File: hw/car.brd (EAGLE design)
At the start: 100 x 80 mm, 27 parts, among them Q1 BS170, Q2 BS170, Q3 BS170, Q4 BS170, Q5 BS170, Q6 BS170, Q7 BS170, Q8 BS170, X0 pwm_board, X1 22-23-2041, X3 22-23-2041

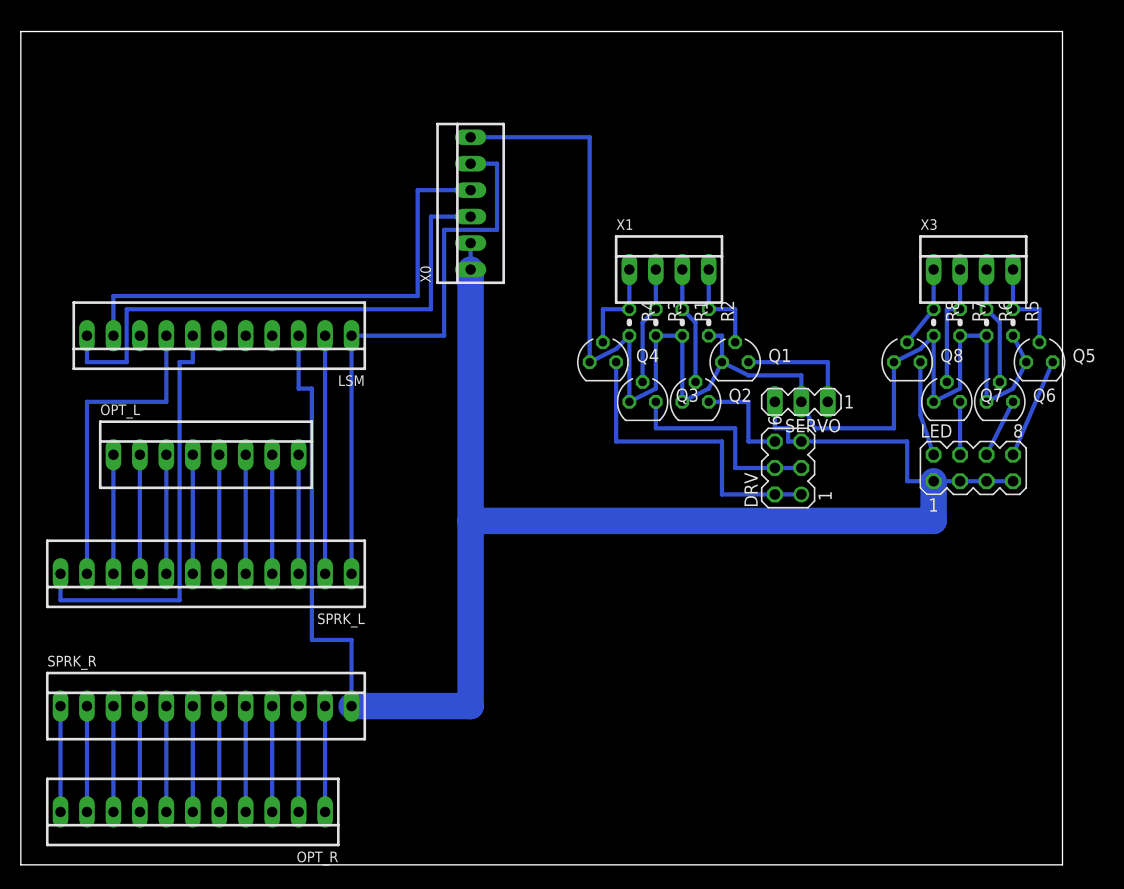
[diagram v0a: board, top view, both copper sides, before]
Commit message: layout v1 done
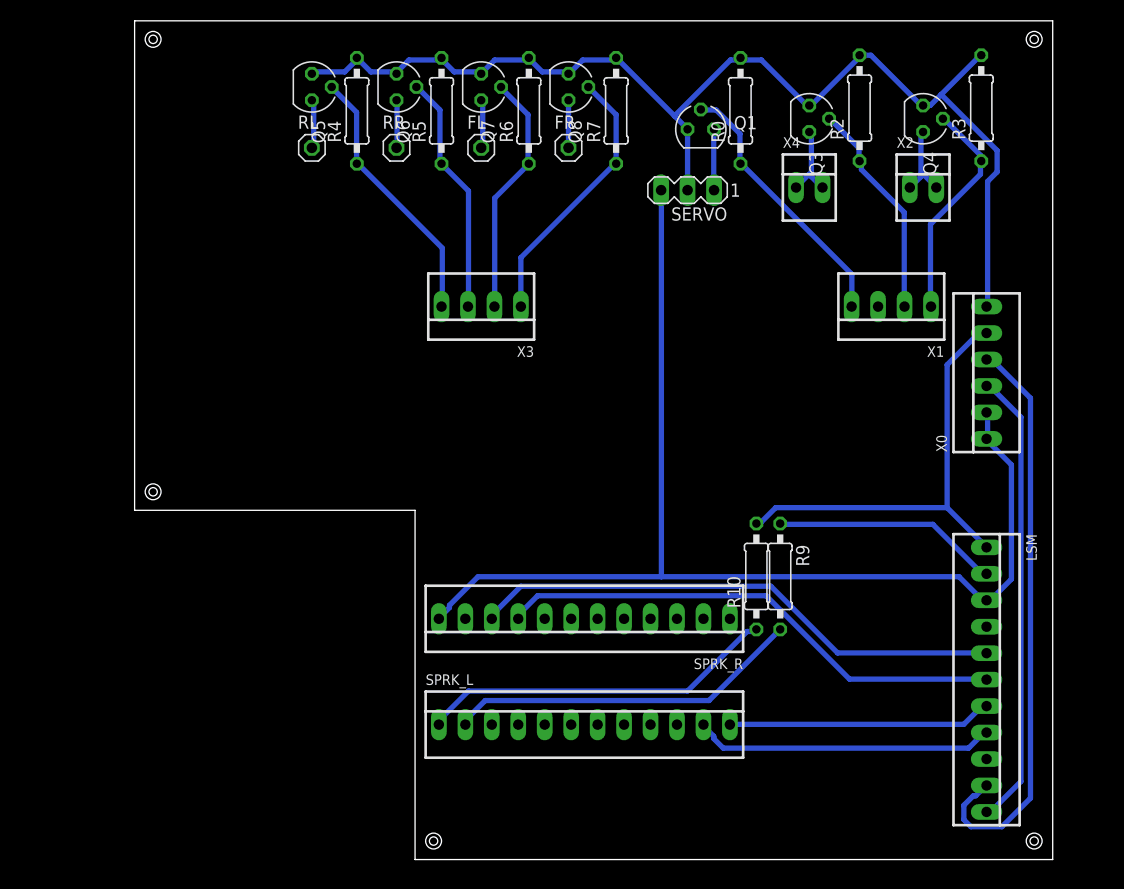
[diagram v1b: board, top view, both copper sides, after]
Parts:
- removed DRV: MTR, con-lstb:MA03-2
- removed LED: 0, con-lstb:MA04-2
- removed OPT_L: 22-23-2081, con-molex:22-23-2081
- removed OPT_R: 22-23-2111, con-molex:22-23-2111
- removed Q2: BS170, transistor-small-signal:SOT54E
- removed R1, R8: 10k, rcl:0204V
- added FL, FR, RL, RR: (no value), pinhead:1X01
- added R0: 10k, rcl:0207/10
- added R10, R9: 0, rcl:0207/10
- added X2, X4: 22-23-2021, con-molex:22-23-2021
- R2, R3, R4, R5, R6, R7: device rcl:0204V -> rcl:0207/10
- moved LSM 80.7 mm to (92.7, 17.8), turned to 270 degrees
- moved Q5 74.7 mm to (27.9, 74.7), turned to 270 degrees
- moved Q6 65.3 mm to (36.1, 74.7), turned to 270 degrees
- moved R5 58.5 mm to (40.4, 72.4), turned to 90 degrees
- moved Q7 54.0 mm to (44.2, 74.7), turned to 270 degrees
- moved X0 52.1 mm to (92.7, 47.2)
- moved R6 48.4 mm to (48.8, 72.4), turned to 90 degrees
- moved X3 47.4 mm to (44.2, 53.6), turned to 180 degrees
- moved Q8 41.9 mm to (52.6, 74.7), turned to 270 degrees
- moved SPRK_L 39.1 mm to (54.1, 13.5), turned to 0 degrees
- moved R7 38.8 mm to (57.1, 72.4), turned to 90 degrees
- moved Q4 38.6 mm to (86.6, 71.6), turned to 270 degrees
- moved R3 37.4 mm to (92.2, 72.6), turned to 90 degrees
- moved SPRK_R 37.3 mm to (54.1, 23.6), turned to 180 degrees
- moved R4 33.1 mm to (32.3, 72.4), turned to 90 degrees
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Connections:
- removed net N$15: LED.6, Q6.S
- removed net N$16: LED.8, Q5.S
- removed net N$23: OPT_L.2, SPRK_L.9
- removed net N$24: OPT_L.3, SPRK_L.8
- removed net N$25: OPT_L.4, SPRK_L.7
- removed net N$26: OPT_L.5, SPRK_L.6
- removed net N$27: OPT_L.6, SPRK_L.5
- removed net N$28: OPT_L.7, SPRK_L.4
- removed net N$29: OPT_L.8, SPRK_L.3
- removed net N$30: OPT_R.11, SPRK_R.1
- removed net N$31: OPT_R.10, SPRK_R.2
- removed net N$32: OPT_R.9, SPRK_R.3
- removed net N$33: OPT_R.8, SPRK_R.4
- removed net N$34: OPT_R.7, SPRK_R.5
- removed net N$35: OPT_R.6, SPRK_R.6
- removed net N$36: OPT_R.5, SPRK_R.7
- removed net N$37: OPT_R.4, SPRK_R.8
- removed net N$40: OPT_R.1, SPRK_R.11
- removed net N$41: DRV.6, Q2.S
- new net 1V8: LSM.2, R9.1
- new net V3V3: LSM.1, R10.2, X0.5
- net GND: no longer DRV.5, LED.1, LED.3, LED.5, LED.7
- net N$1: now also R0.1; no longer R2.1
- net N$10: now also R4.1; no longer R5.1
- net N$11: now also R5.1; no longer R6.1
- net N$12: now also R6.1; no longer R7.1
- net N$13: now also R7.1; no longer R8.1
- net N$14: now also FL.1; no longer LED.4
- net N$17: now also R9.2; no longer LSM.2
- net N$2: now also Q4.S, X2.1, X2.2; no longer Q2.G, R1.1, X1.3
- net N$22: now also R10.1, SPRK_L.1; no longer OPT_L.1, SPRK_L.10
- net N$3: now also R2.1; no longer R3.1
- net N$38: now also LSM.6; no longer OPT_R.3
- net N$39: now also LSM.5; no longer OPT_R.2
- net N$4: now also R3.1; no longer R4.1
- net N$6: now also Q5.S, RL.1; no longer DRV.1, DRV.2, Q4.S
- net N$7: now also Q6.S, RR.1; no longer DRV.3, DRV.4, Q3.S
- net N$8: now also Q3.S, X4.1, X4.2; no longer LSM.1, SPRK_L.1, X0.5
- net N$9: now also FR.1; no longer LED.2
- net VM: now also R0.2; no longer Q2.D, R1.2, R8.2
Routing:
- net GND: track 175.3 -> 112.9 mm
- net N$8: track 55.9 -> 7.88 mm
- net V3V3: track 0.00 -> 43.1 mm
- net N$39: track 10.2 -> 51.8 mm
- net N$38: track 10.2 -> 49.6 mm
- net N$6: track 30.5 -> 4.79 mm
- net N$22: track 11.4 -> 34.5 mm
- net 1V8: track 0.00 -> 21.9 mm
- net VM: track 133.9 -> 112.8 mm
- net N$13: track 7.88 -> 26.2 mm
- net N$1: track 9.52 -> 25.9 mm
- net N$10: track 9.53 -> 25.7 mm
- net N$7: track 20.3 -> 4.61 mm
- net N$21: track 40.6 -> 25.4 mm
- net N$4: track 9.52 -> 21.7 mm
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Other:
- board size 100 x 80 mm -> 88.1 x 80.5 mm
